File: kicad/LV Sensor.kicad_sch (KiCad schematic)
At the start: 42 parts, among them U1 MCP2518FD-xJHA, U10 FT231XS-R, U2 AP63203WU-7, U3 XMSM0C1104SPW20R, U4 AP63205WU-7, U5 ATA6561-GAQW-N, U6 DSC1001DL5, U7 ADS114S06BIPBSR, U8 LM2662MX/NOPB, U9 TLV77325PDBVR

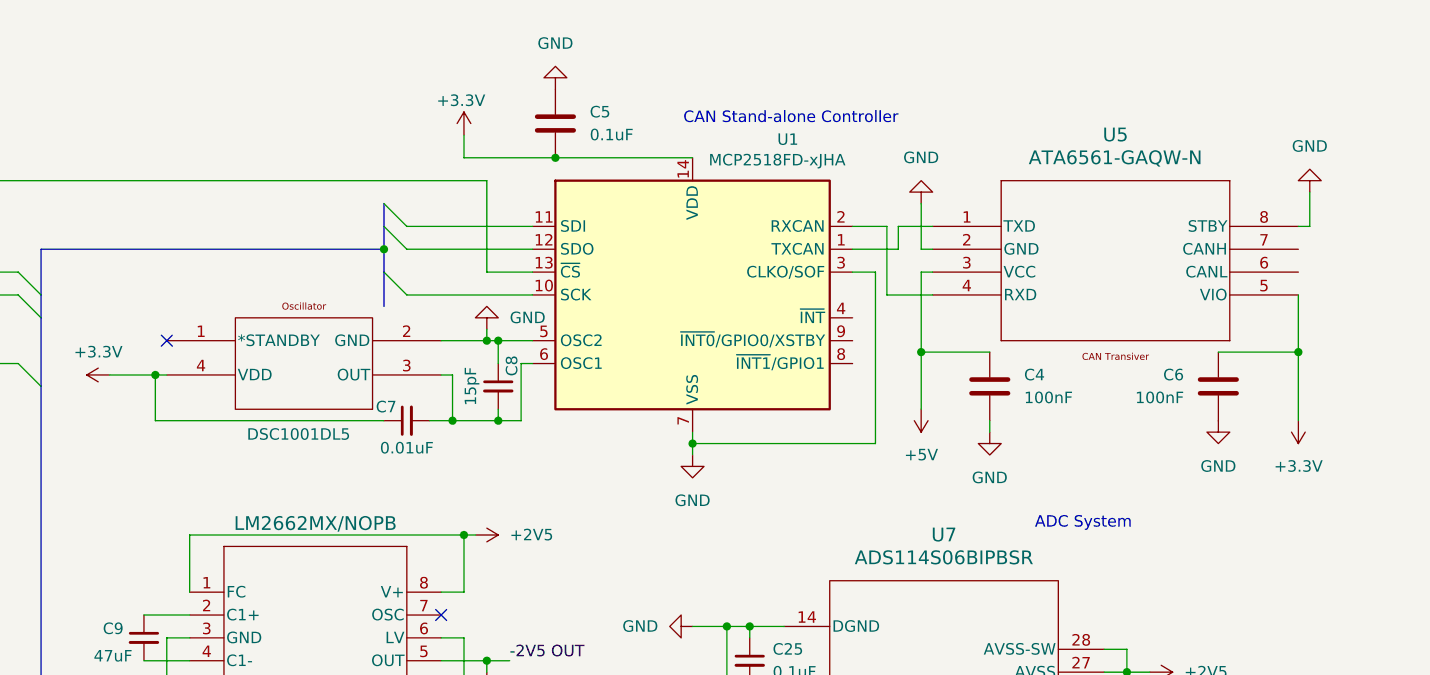
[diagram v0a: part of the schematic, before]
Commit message: 09-06-2025 Fixed Some Changes
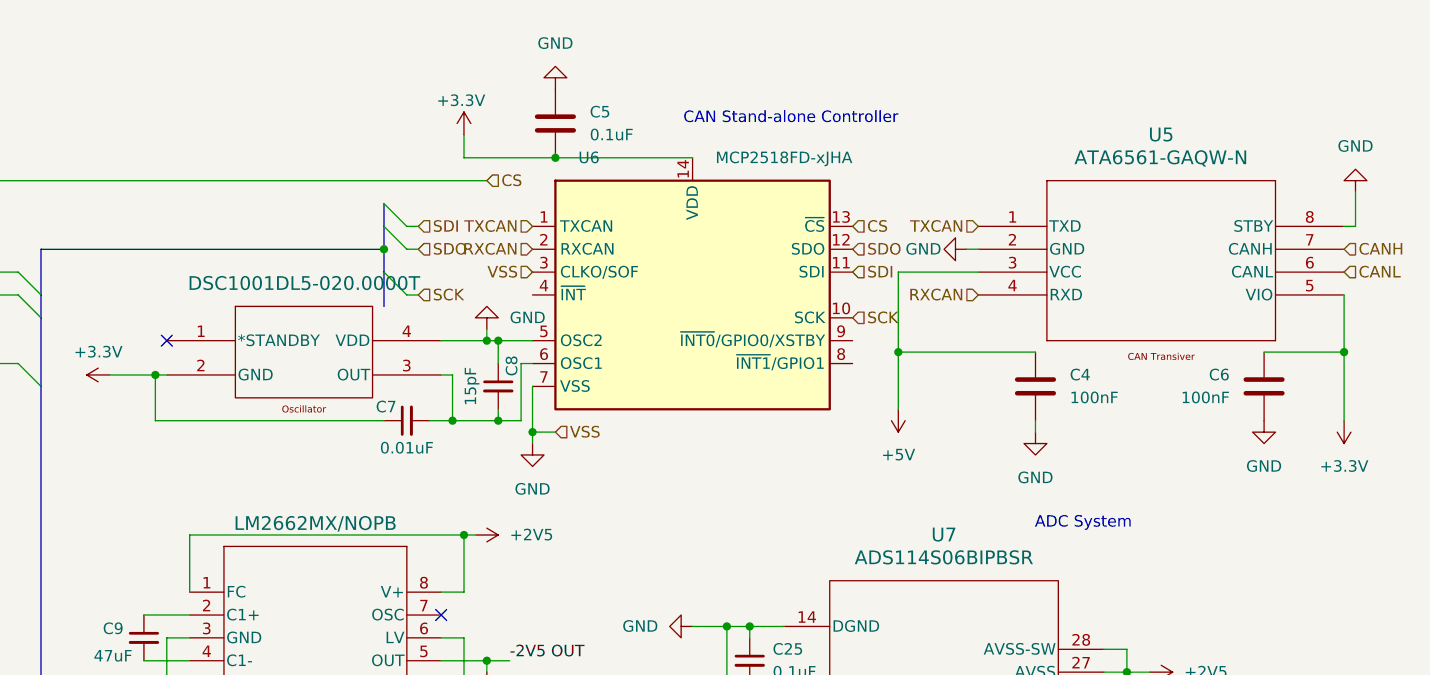
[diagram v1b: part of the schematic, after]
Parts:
- removed U1: MCP2518FD-xJHA, LV-Sensor-Footprints-Lib:MCP2518FDT, symbol LV-Sensor-Lib:MCP2517FD-xJHA
- removed U6: DSC1001DL5, LV-Sensor-Footprints-Lib:CDFN4_2P5X2_MCH, symbol LV-Sensor-Lib:DSC1001DL5-020.0000T
- added U11: DSC1001DL5-020.0000T, LV-Sensor-Footprints-Lib:CDFN4_2P5X2_MCH, symbol LV-Sensor-Lib:DSC1001DL5-020.0000T
- added U6: MCP2518FD-xJHA, LV-Sensor-Footprints-Lib:MCP2518FDT, symbol LV-Sensor-Lib:MCP2517FD-xJHA
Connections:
- net +3.3V: now also U11.2 (GND), U6.14 (VDD)
- net GND: now also U11.4 (VDD), U6.3 (CLKO/SOF), U6.5 (OSC2), U6.7 (VSS)
- net TXCAN: now reaches U5.1 (TXD)
- net TXCAN: now also U6.1 (TXCAN)
- net RXCAN: now reaches U5.4 (RXD)
- net RXCAN: now also U6.2 (RXCAN)
- net CANL: now reaches U5.6 (CANL)
- net CANH: now reaches U5.7 (CANH)
- net at C7.2, C8.2: now also U11.3 (OUT), U6.6 (OSC1)
- net CS: now reaches U3.8 (PA2)
- net CS: now also U6.13 (~{CS})
- new net SCK: U6.10 (SCK)
- new net SDI: U6.11 (SDI)
- new net SDO: U6.12 (SDO)
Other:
- moved on the sheet: C4, C6, U5

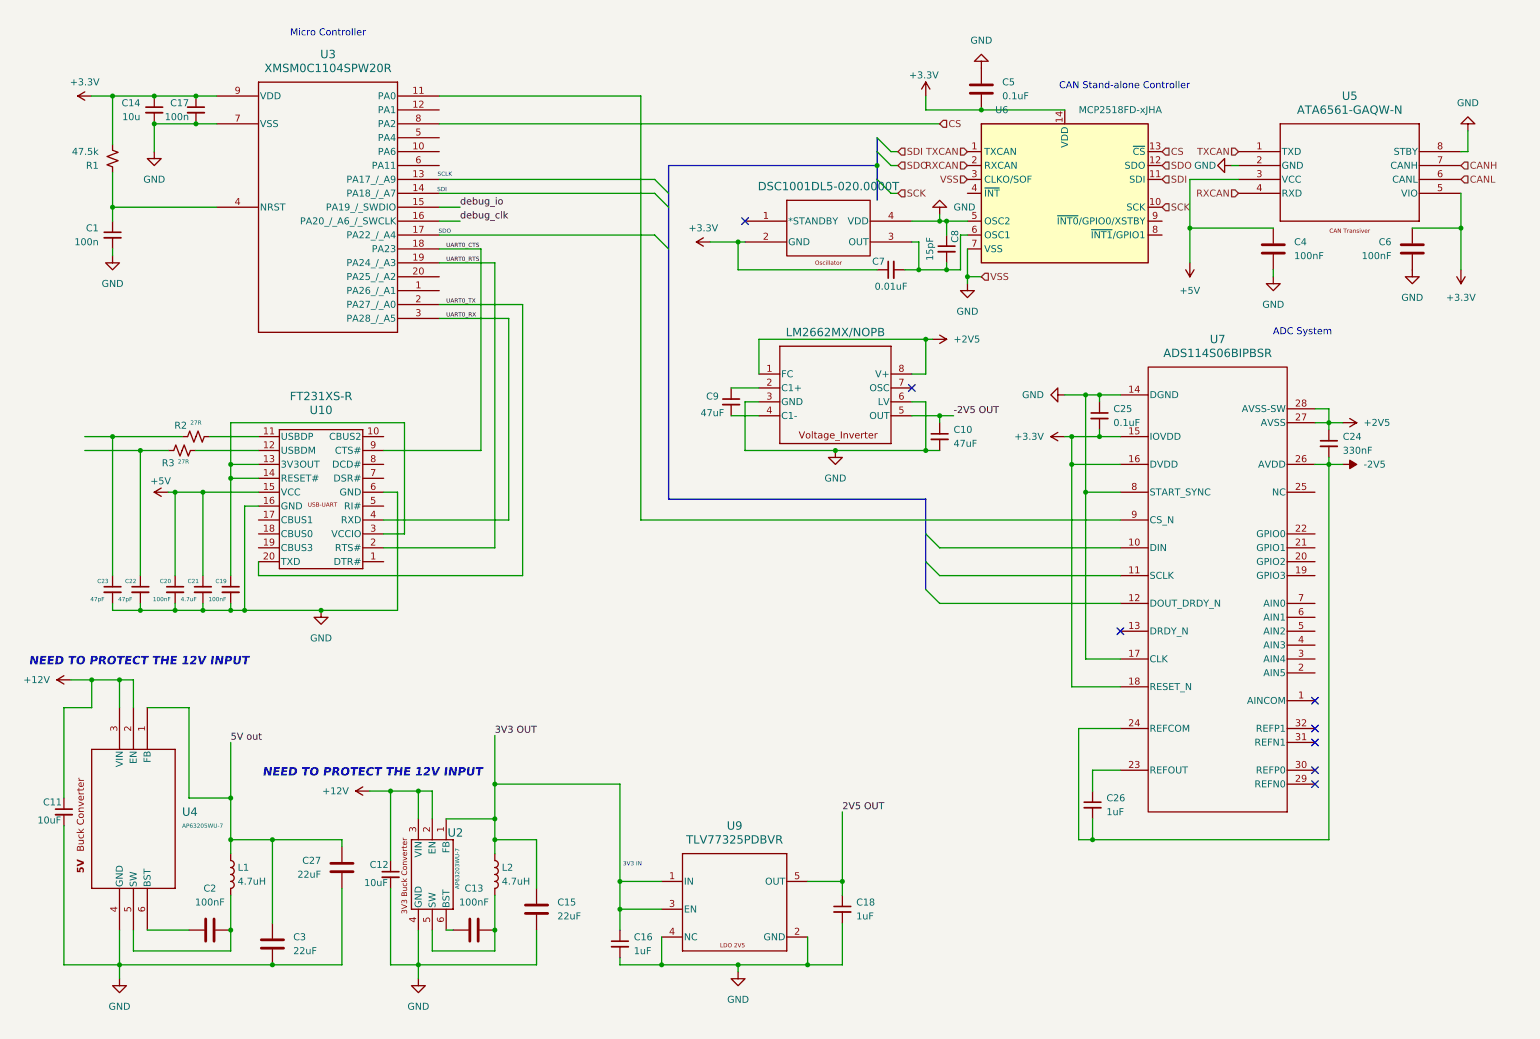
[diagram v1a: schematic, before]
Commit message: 09-06-2025 Again
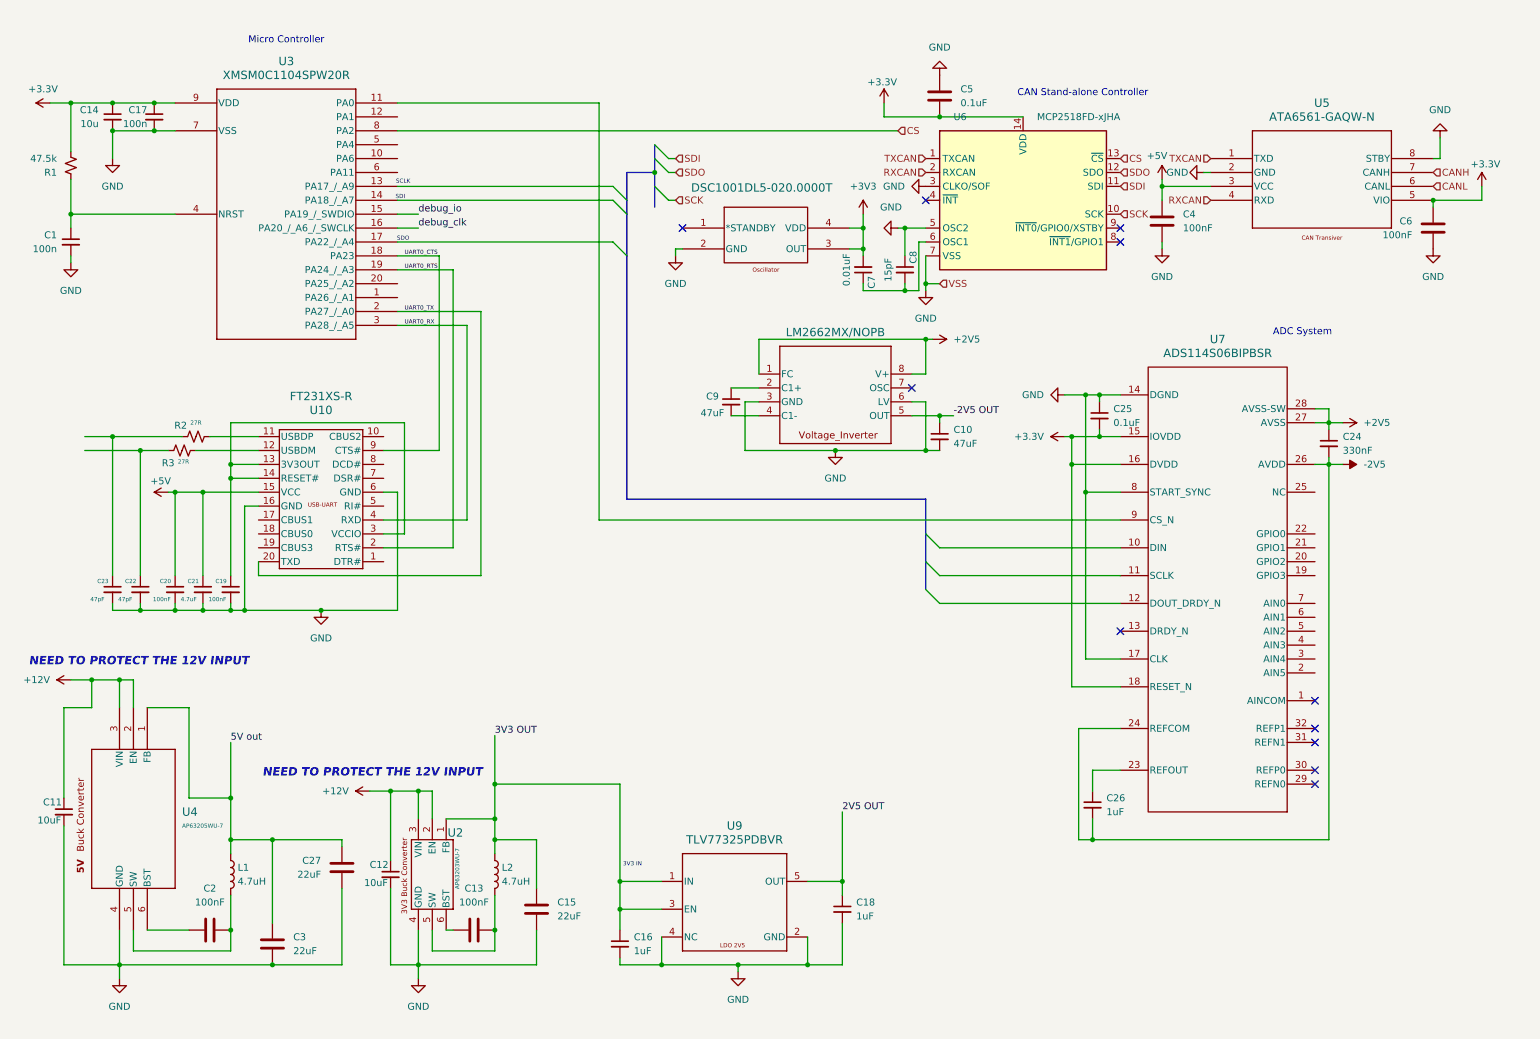
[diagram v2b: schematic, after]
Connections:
- net +3.3V: no longer C7.1, U11.2 (GND)
- net GND: now also U11.2 (GND); no longer U11.4 (VDD)
- net at C8.2, U6.6 (OSC1): now also C7.1; no longer C7.2, U11.3 (OUT)
- new net +3V3: C7.2, U11.3 (OUT), U11.4 (VDD)
- no-connect marks 8 -> 11
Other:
- moved on the sheet: C1, C14, C17, C4, C5, C6, C7, C8, R1, U3, U5, U6

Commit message: 09-26-2005
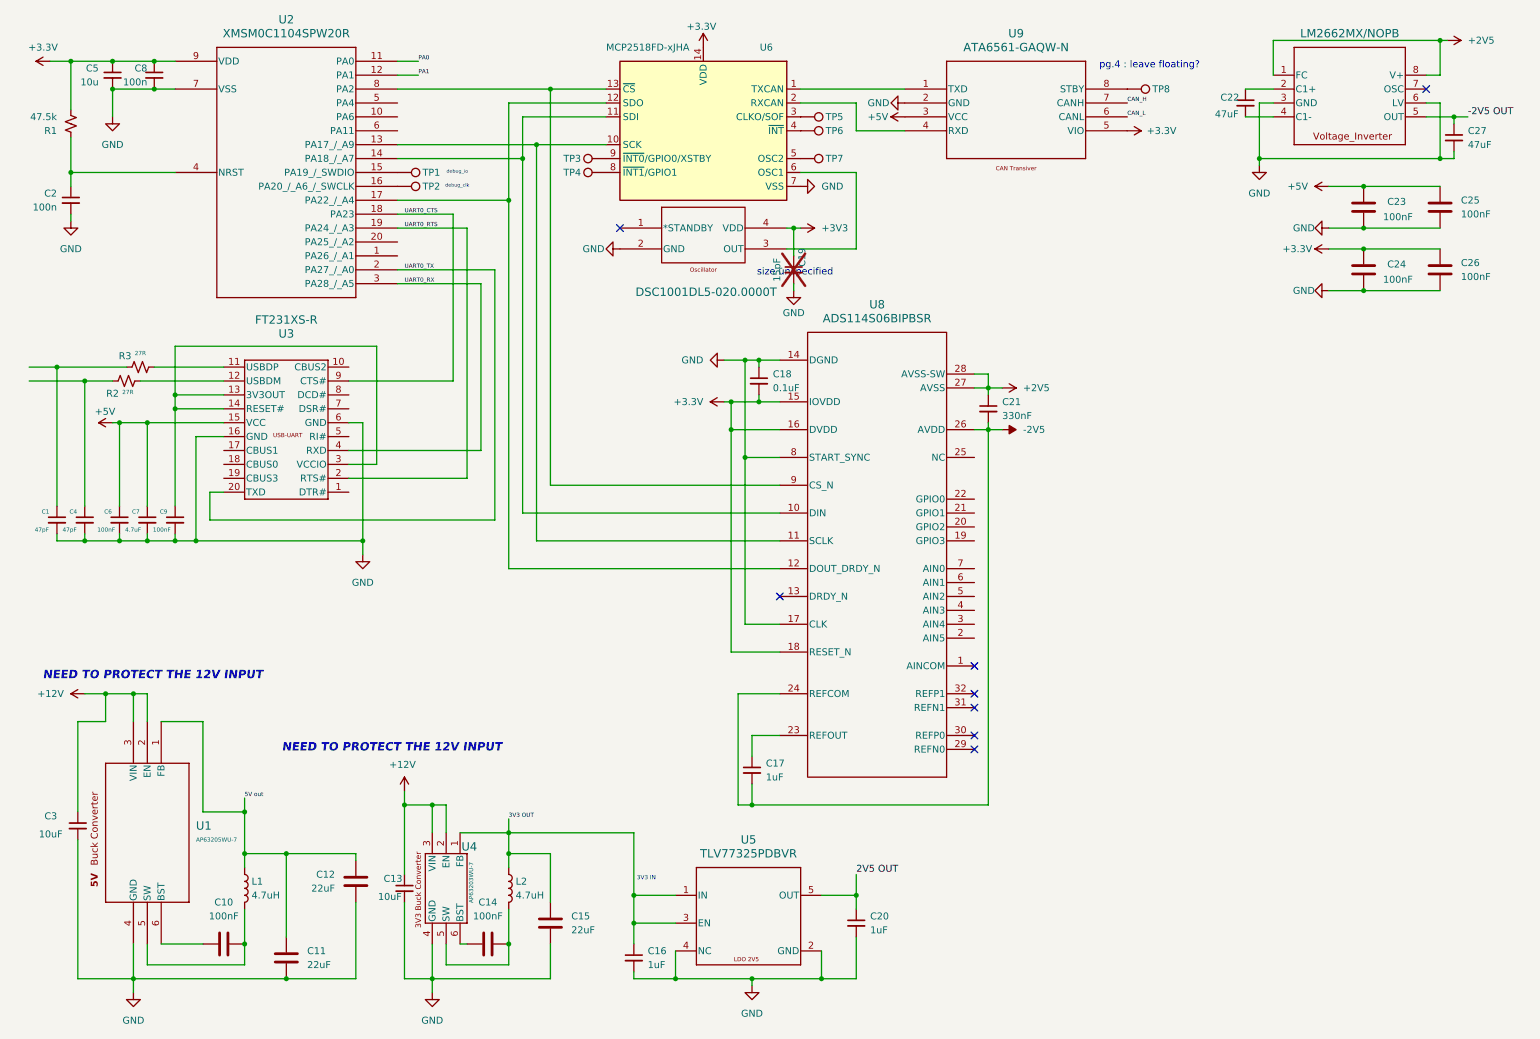
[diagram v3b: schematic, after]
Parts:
- removed C5: 0.1uF, Capacitor_SMD:C_1206_3216Metric_Pad1.33x1.80mm_HandSolder, symbol Device:C
- removed C7: 0.01uF, Capacitor_SMD:C_1206_3216Metric_Pad1.33x1.80mm_HandSolder, symbol Device:C_Small
- added C23, C25: 100nF, Capacitor_SMD:C_1206_3216Metric_Pad1.33x1.80mm_HandSolder, symbol Device:C
- added TP1, TP2, TP3, TP4, TP5, TP6, TP7, TP8: TestPoint, symbol Connector:TestPoint
- C19: renamed from C8; now not fitted; now left out of the parts list
- renumbered C23 to C1, C2 to C10, C3 to C11, C27 to C12, C12 to C13, C13 to C14, C26 to C17, C25 to C18, C1 to C2, C18 to C20, C24 to C21, C9 to C22, C4 to C24, C6 to C26, C10 to C27, C11 to C3, C22 to C4, C14 to C5, C20 to C6, C21 to C7, C17 to C8, C19 to C9, R3 to R2, R2 to R3, U4 to U1, U8 to U10, U3 to U2, U10 to U3, U2 to U4, U9 to U5, U11 to U7, U7 to U8, U5 to U9
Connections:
- net CS is gone; now on an unnamed net: U2.8 (PA2), U6.13 (~{CS})
- net SCK is gone; now on an unnamed net: U6.10 (SCK)
- net SDI is gone; now on an unnamed net: U6.11 (SDI)
- net SDO is gone; now on an unnamed net: U6.12 (SDO)
- net +3.3V: now also C24.1
- net +3V3: now also C19.1; no longer U7.3 (OUT)
- net +5V: now also C23.1, C25.1; no longer C24.1
- net GND: now also C19.2, C23.2, C25.2; no longer C19.1, U6.3 (CLKO/SOF), U6.5 (OSC2), U9.8 (STBY)
- net at U8.10 (DIN): now also U2.14 (PA18_/_A7)
- net at U8.11 (SCLK): now also U2.13 (PA17_/_A9)
- net at U8.12 (DOUT_DRDY_N): now also U2.17 (PA22_/_A4)
- net at U8.9 (CS_N): no longer U2.11 (PA0)
- net at U6.6 (OSC1): now also U7.3 (OUT); no longer C19.2
- net PA1: now reaches U2.12 (PA1)
- net at U6.4 (~{INT}): now also TP6.1
- net at U6.8 (~{INT1}/GPIO1): now also TP4.1
- net at U6.9 (~{INT0}/GPIO0/XSTBY): now also TP3.1
- net CANH renamed CAN_H
- net CANL renamed CAN_L
- net RXCAN: no longer names the net of U6.2 (RXCAN), U9.4 (RXD)
- net TXCAN: no longer names the net of U6.1 (TXCAN), U9.1 (TXD)
- net debug_clk: no longer names the net of U2.16 (PA20_/_A6_/_SWCLK)
- net debug_clk: now also TP2.1
- net debug_io: no longer names the net of U2.15 (PA19_/_SWDIO)
- net debug_io: now also TP1.1
- new net: TP5.1, U6.3 (CLKO/SOF)
- new net: TP8.1, U9.8 (STBY)
- new net: TP7.1, U6.5 (OSC2)
- new net PA0: U2.11 (PA0)
- no-connect marks 11 -> 8
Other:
- note added: "debug_clk"
- note added: "debug_io"
- note added: "pg.4 : leave floating?"
- note added: "size unspecified"
- note removed: "ADC System"
- note removed: "CAN Stand-alone Controller"
- note removed: "Micro Controller"
- note removed: "SCLK"
- note removed: "SDI"
- note removed: "SDO"
- moved on the sheet: C1, C10, C11, C12, C13, C14, C15, C16, C17, C18, C2, C20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
